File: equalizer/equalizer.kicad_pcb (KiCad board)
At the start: 2 copper layers, 35 parts, among them U105 TL072, U106 TL072

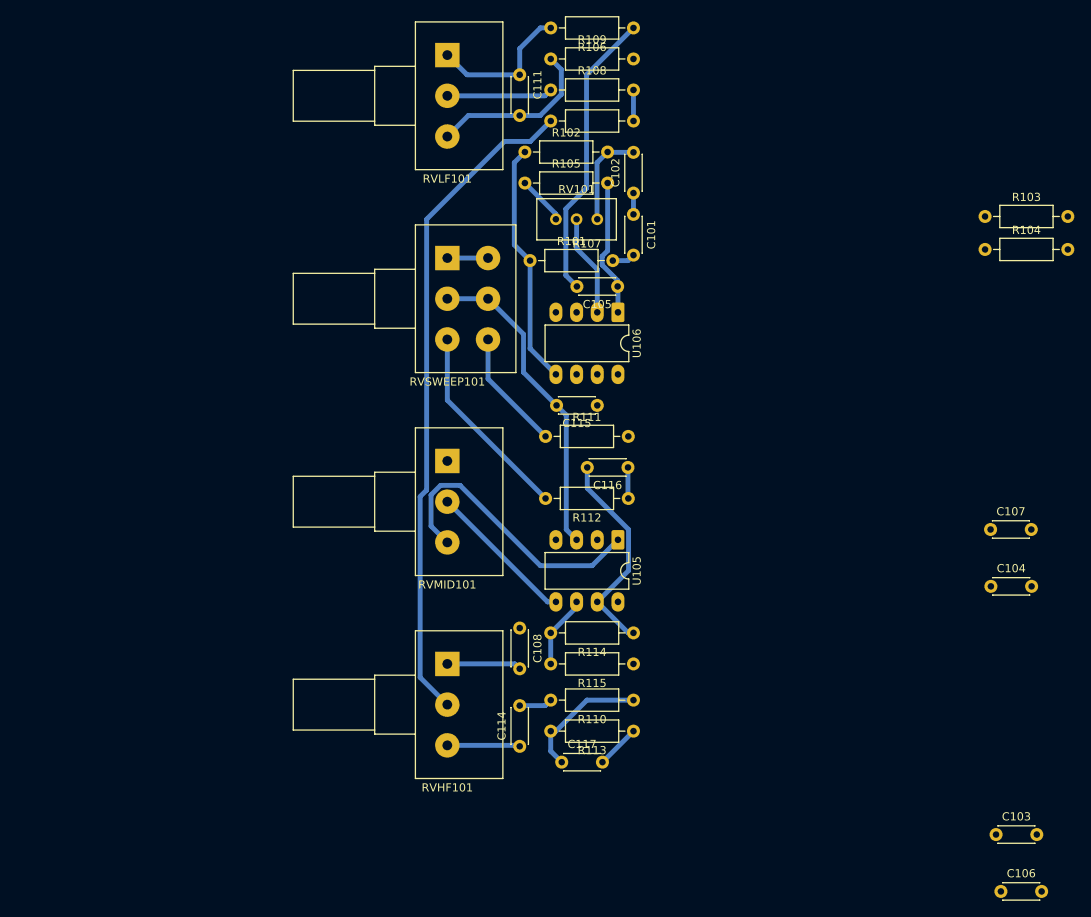
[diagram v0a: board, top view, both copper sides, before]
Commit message: before breaking everything
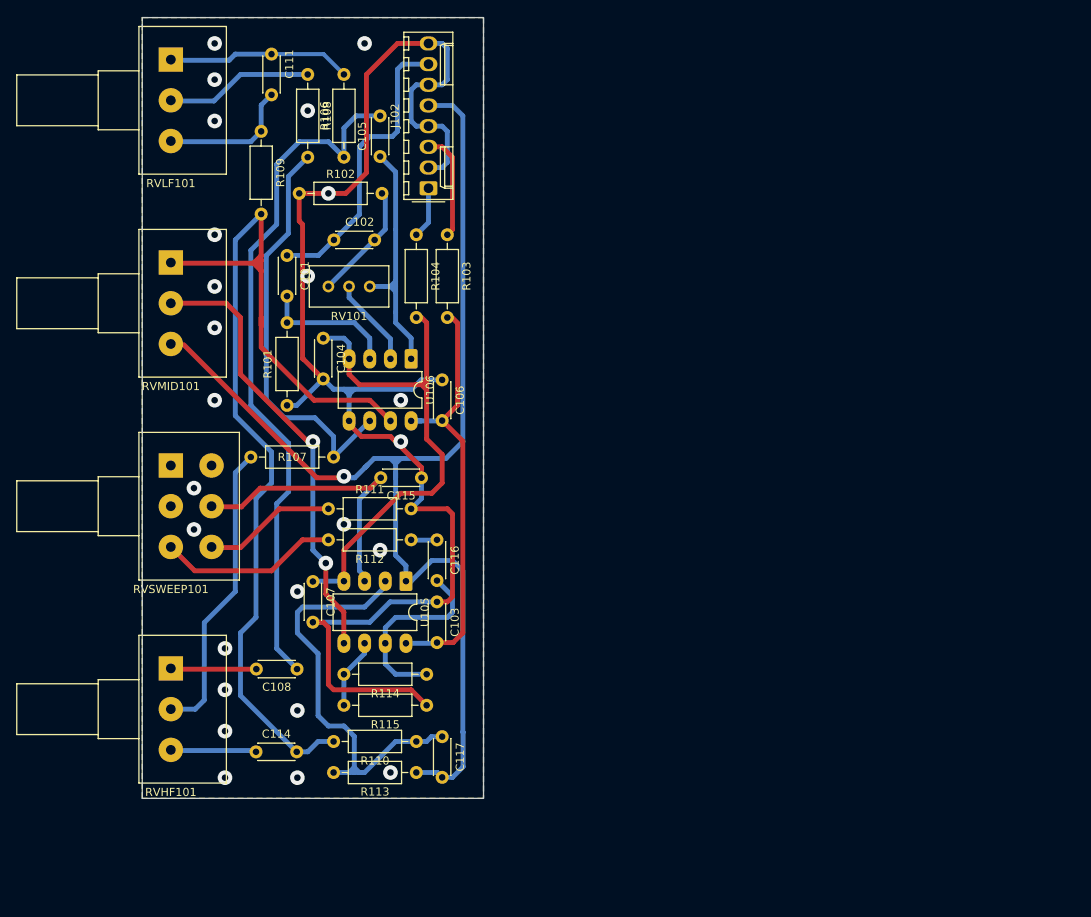
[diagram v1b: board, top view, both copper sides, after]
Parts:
- removed R105: 4k7, Resistor_THT:R_Axial_DIN0207_L6.3mm_D2.5mm_P10.16mm_Horizontal
- added J102: Conn_01x08_Socket, Connector_Molex:Molex_KK-254_AE-6410-08A_1x08_P2.54mm_Vertical, F.Cu at (189.5, 48.3)
- moved C106 93.0 mm to (191.1, 71.8), turned to -90 degrees
- moved C104 87.5 mm to (176.5, 66.7), turned to -90 degrees
- moved C107 83.5 mm to (175.3, 96.6), turned to -90 degrees
- moved C103 74.4 mm to (190.5, 99.1), turned to -90 degrees
- moved R104 69.9 mm to (188.0, 54.0), turned to -90 degrees
- moved R103 66.1 mm to (191.8, 54.0), turned to -90 degrees
- moved R107 55.3 mm to (177.8, 81.3)
- moved C101 42.8 mm to (172.1, 56.5)
- moved RVSWEEP101 42.5 mm to (157.8, 82.3)
- moved RVMID101 41.8 mm to (157.8, 57.4)
- moved R106 38.9 mm to (179.1, 44.5), turned to 90 degrees
- moved C102 37.2 mm to (177.8, 54.6), turned to 0 degrees
- moved R109 36.7 mm to (168.9, 41.3), turned to -90 degrees
- moved R101 34.7 mm to (172.1, 74.9), turned to 90 degrees
- moved RV101 34.0 mm to (177.2, 60.3), turned to 180 degrees
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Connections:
- net /IN renamed IN
- net /OUT renamed OUT
- RV101 pad 3: Net-(R105-Pad1) -> Net-(C105-Pad1)
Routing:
- net GND: track 30.0 -> 180.9 mm, vias 0 -> 25
- net Net-(C114-Pad2): track 4.09 -> 129.3 mm
- net OUT: track 40.9 -> 144.8 mm, vias 0 -> 1
- net Net-(U105C-V-): track 0.00 -> 64.8 mm
- net Net-(U105C-V+): track 0.00 -> 53.4 mm
- net Net-(C105-Pad2): track 35.8 -> 85.8 mm
- net Net-(U106B--): track 3.81 -> 50.8 mm
- net Net-(R107-Pad2): track 81.6 -> 36.8 mm
- net Net-(U105A--): track 16.1 -> 52.8 mm
- net Net-(U105B-+): track 18.4 -> 54.9 mm, vias 0 -> 2
- net IN: track 2.62 -> 36.4 mm
- net Net-(C105-Pad1): track 17.0 -> 31.4 mm
- net Net-(U106A-+): track 2.82 -> 16.7 mm
- net +12V: track 0.00 -> 13.3 mm
- net -12V: track 0.00 -> 6.34 mm
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- added copper zone on B.Cu, net GND
- added copper zone on F.Cu, net GND
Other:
- board outline added: 41.9 x 95.9 mm
